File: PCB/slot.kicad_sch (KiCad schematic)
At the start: 3 parts, among them J8 EdgeConn_Full

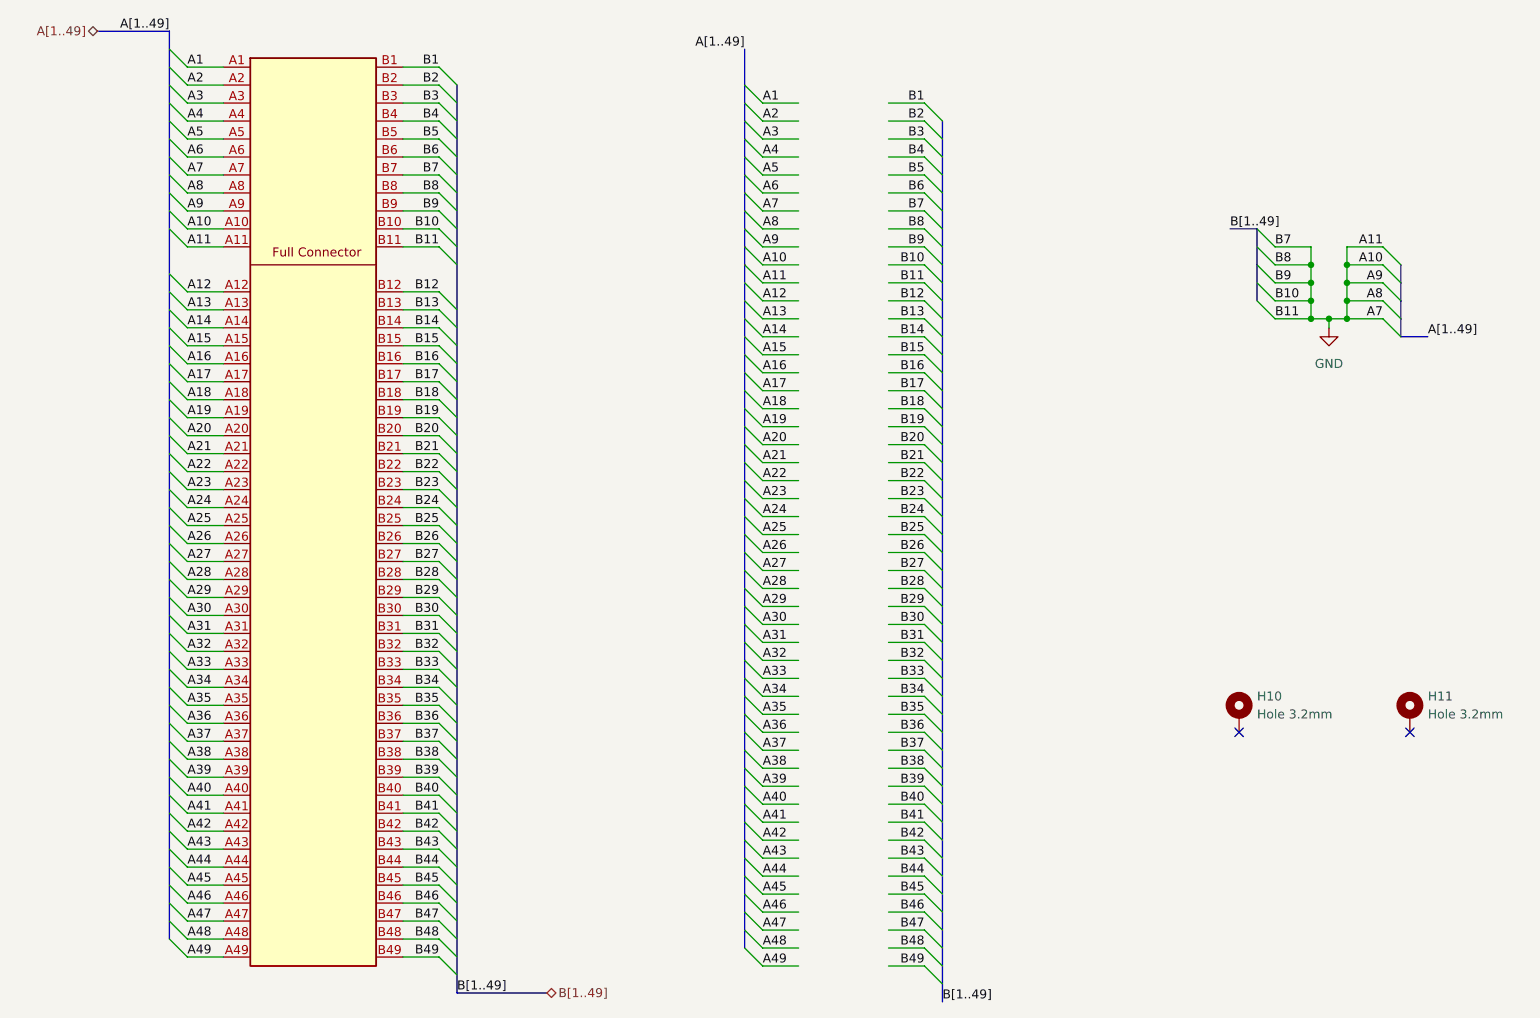
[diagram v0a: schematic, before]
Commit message: Traced ethernet
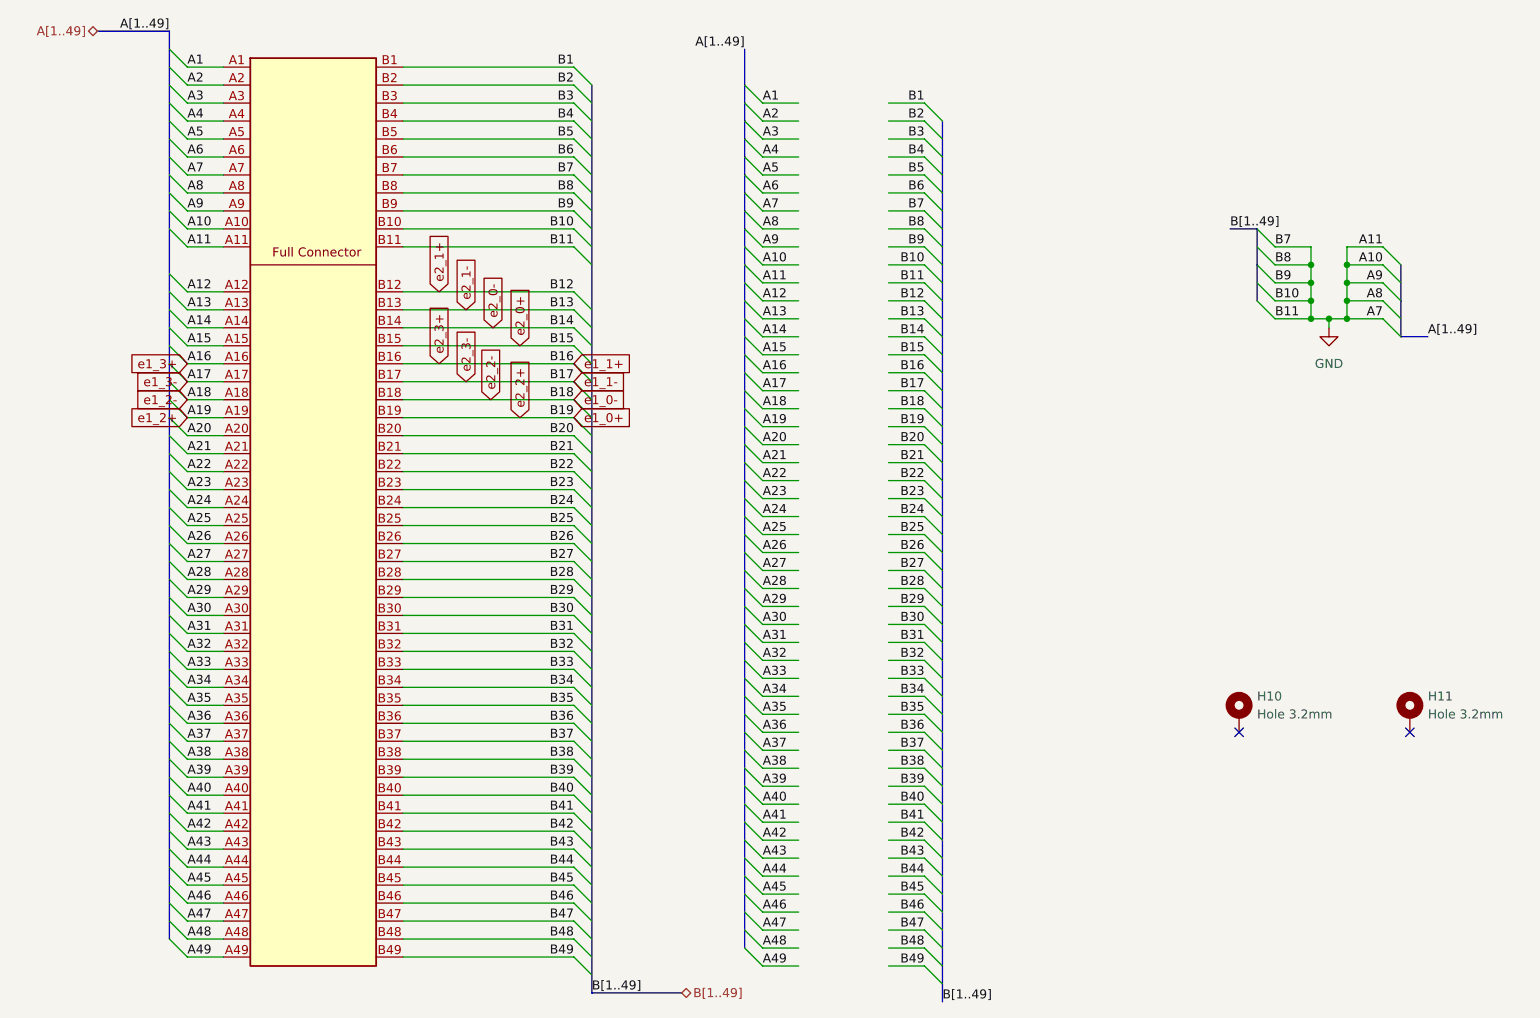
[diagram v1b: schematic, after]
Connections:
- net A16 renamed e1_3+
- net A17 renamed e1_3-
- net A18 renamed e1_2-
- net A19 renamed e1_2+
- net B12 renamed e2_1+
- net B13 renamed e2_1-
- net B14 renamed e2_0-
- net B15 renamed e2_0+
- net B16 renamed e1_1+
- net B17 renamed e1_1-
- net B18 renamed e1_0-
- net B19 renamed e1_0+
